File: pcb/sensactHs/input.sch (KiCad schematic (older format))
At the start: 5 parts, among them U18 PCA9555, U19 PCA9555

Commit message: new version of sensactHs
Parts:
- removed INP4: ROTENC, Pin_Headers:Pin_Header_Straight_1x05, symbol CONN_01X05
- added C1, C2, C3, C4: u1, Capacitors_SMD:C_0805_HandSoldering, symbol C
- added INP3: PUSH_BUTTON_INPUT, w_conn_strip:vasch_strip_17x2, symbol CONN_01X34
- added U3, U4: PCA9555, sensact:TSSOP-24_4.4x7.8mm_Pitch0.65mm_handsolder, symbol PCA9555
- U1: renamed from U19; footprint kl_footprints:TSSOP-24_4.4x7.8mm_Pitch0.65mm_handsolder -> sensact:TSSOP-24_4.4x7.8mm_Pitch0.65mm_handsolder
- U2: renamed from U18; footprint kl_footprints:TSSOP-24_4.4x7.8mm_Pitch0.65mm_handsolder -> sensact:TSSOP-24_4.4x7.8mm_Pitch0.65mm_handsolder
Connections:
- net labels removed: PB6, PB7, PC13
- wire segments 241 -> 463
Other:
- moved on the sheet: INP2

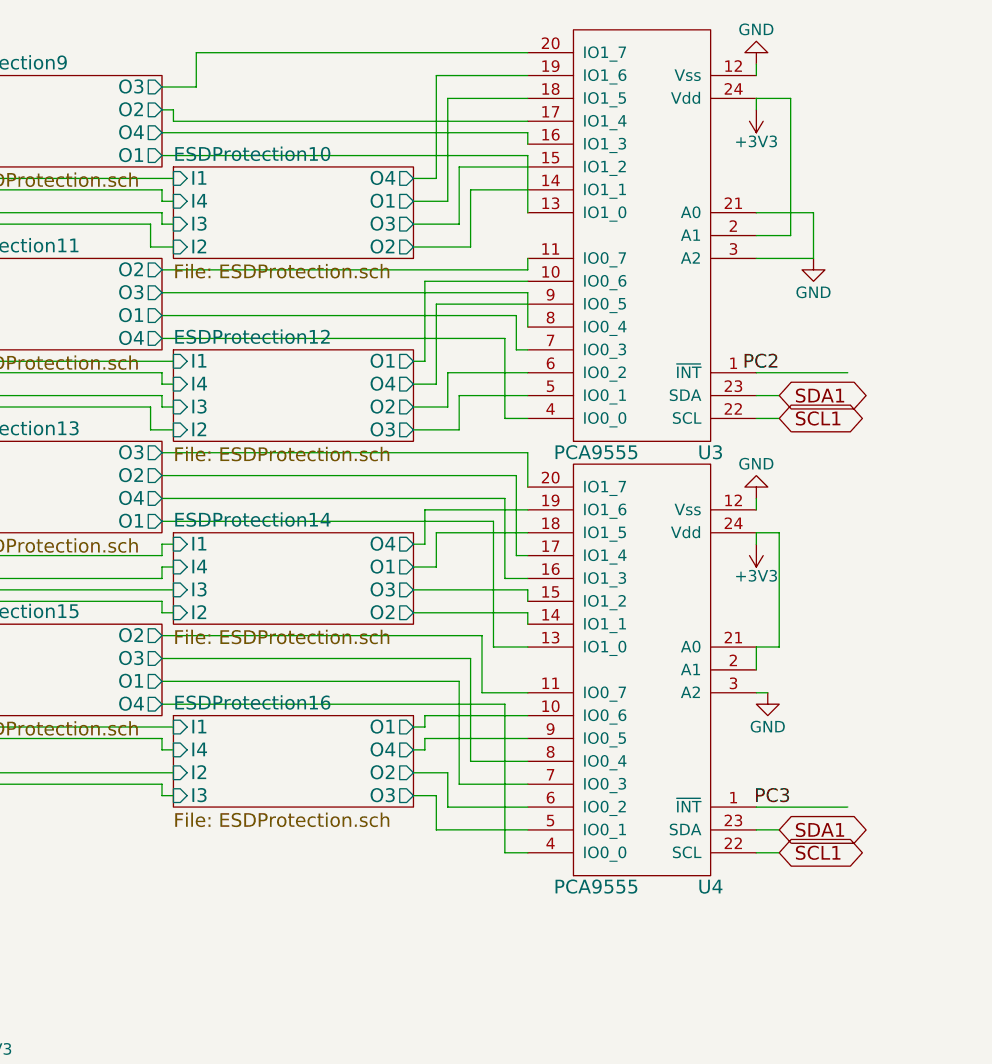
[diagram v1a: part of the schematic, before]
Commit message: sensactHS intermediate backup
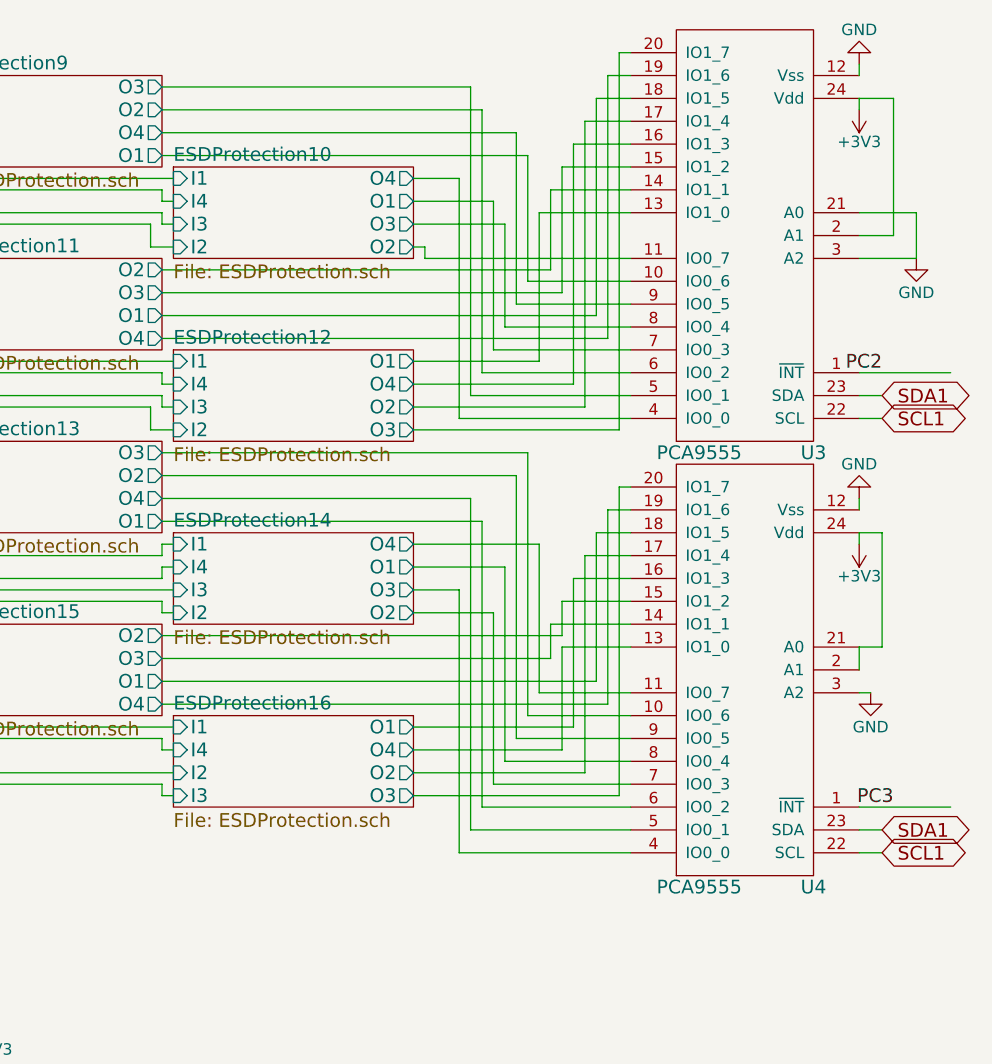
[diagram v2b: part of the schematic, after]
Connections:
- net ESDProtection10/O1: now also U3.7 (IO0_3); no longer U3.18 (IO1_5)
- net ESDProtection10/O2: now also U3.11 (IO0_7); no longer U3.14 (IO1_1)
- net ESDProtection10/O3: now also U3.8 (IO0_4); no longer U3.15 (IO1_2)
- net ESDProtection10/O4: now also U3.4 (IO0_0); no longer U3.19 (IO1_6)
- net ESDProtection11/O1: now also U3.18 (IO1_5); no longer U3.7 (IO0_3)
- net ESDProtection11/O2: now also U3.14 (IO1_1); no longer U3.11 (IO0_7)
- net ESDProtection11/O3: now also U3.15 (IO1_2); no longer U3.8 (IO0_4)
- net ESDProtection11/O4: now also U3.19 (IO1_6); no longer U3.4 (IO0_0)
- net ESDProtection12/O1: now also U3.13 (IO1_0); no longer U3.10 (IO0_6)
- net ESDProtection12/O2: now also U3.17 (IO1_4); no longer U3.6 (IO0_2)
- net ESDProtection12/O3: now also U3.20 (IO1_7); no longer U3.5 (IO0_1)
- net ESDProtection12/O4: now also U3.16 (IO1_3); no longer U3.9 (IO0_5)
- net ESDProtection13/O1: now also U4.6 (IO0_2); no longer U4.13 (IO1_0)
- net ESDProtection13/O2: now also U4.9 (IO0_5); no longer U4.17 (IO1_4)
- net ESDProtection13/O3: now also U4.10 (IO0_6); no longer U4.20 (IO1_7)
- net ESDProtection13/O4: now also U4.5 (IO0_1); no longer U4.16 (IO1_3)
- net ESDProtection14/O1: now also U4.8 (IO0_4); no longer U4.18 (IO1_5)
- net ESDProtection14/O2: now also U4.7 (IO0_3); no longer U4.14 (IO1_1)
- net ESDProtection14/O3: now also U4.4 (IO0_0); no longer U4.15 (IO1_2)
- net ESDProtection14/O4: now also U4.11 (IO0_7); no longer U4.19 (IO1_6)
- net ESDProtection15/O1: now also U4.18 (IO1_5); no longer U4.7 (IO0_3)
- net ESDProtection15/O2: now also U4.15 (IO1_2); no longer U4.11 (IO0_7)
- net ESDProtection15/O3: now also U4.14 (IO1_1); no longer U4.8 (IO0_4)
- net ESDProtection15/O4: now also U4.19 (IO1_6); no longer U4.4 (IO0_0)
- net ESDProtection16/O1: now also U4.16 (IO1_3); no longer U4.10 (IO0_6)
- net ESDProtection16/O2: now also U4.17 (IO1_4); no longer U4.6 (IO0_2)
- net ESDProtection16/O3: now also U4.20 (IO1_7); no longer U4.5 (IO0_1)
- net ESDProtection16/O4: now also U4.13 (IO1_0); no longer U4.9 (IO0_5)
- net ESDProtection9/O1: now also U3.10 (IO0_6); no longer U3.13 (IO1_0)
- net ESDProtection9/O2: now also U3.6 (IO0_2); no longer U3.17 (IO1_4)
- net ESDProtection9/O3: now also U3.5 (IO0_1); no longer U3.20 (IO1_7)
- net ESDProtection9/O4: now also U3.9 (IO0_5); no longer U3.16 (IO1_3)
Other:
- moved on the sheet: U3, U4
